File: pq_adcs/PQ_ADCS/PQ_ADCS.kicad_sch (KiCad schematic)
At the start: 55 parts, among them J1 CES-110-02-L-S, J10 Pico-Clasp_01x09, J11 Pico-Clasp_01x15, J12 CES-102-02-L-S, J2 CES-110-02-L-S, J3 CES-110-02-L-S, J4 CES-110-02-L-S, J5 Pico-Clasp_01x02, J6 Pico-Clasp_01x10, J7 Pico-Clasp_01x10, J8 Pico-Clasp_01x10, J9 Pico-Clasp_01x10, U1 LPV542, U2 LPV542, U3 LPV542, U4 IIM-42652, U5 TLC59208FIRGYR, U6 TMUX1108RSVR, U7 TCN75AVOA713

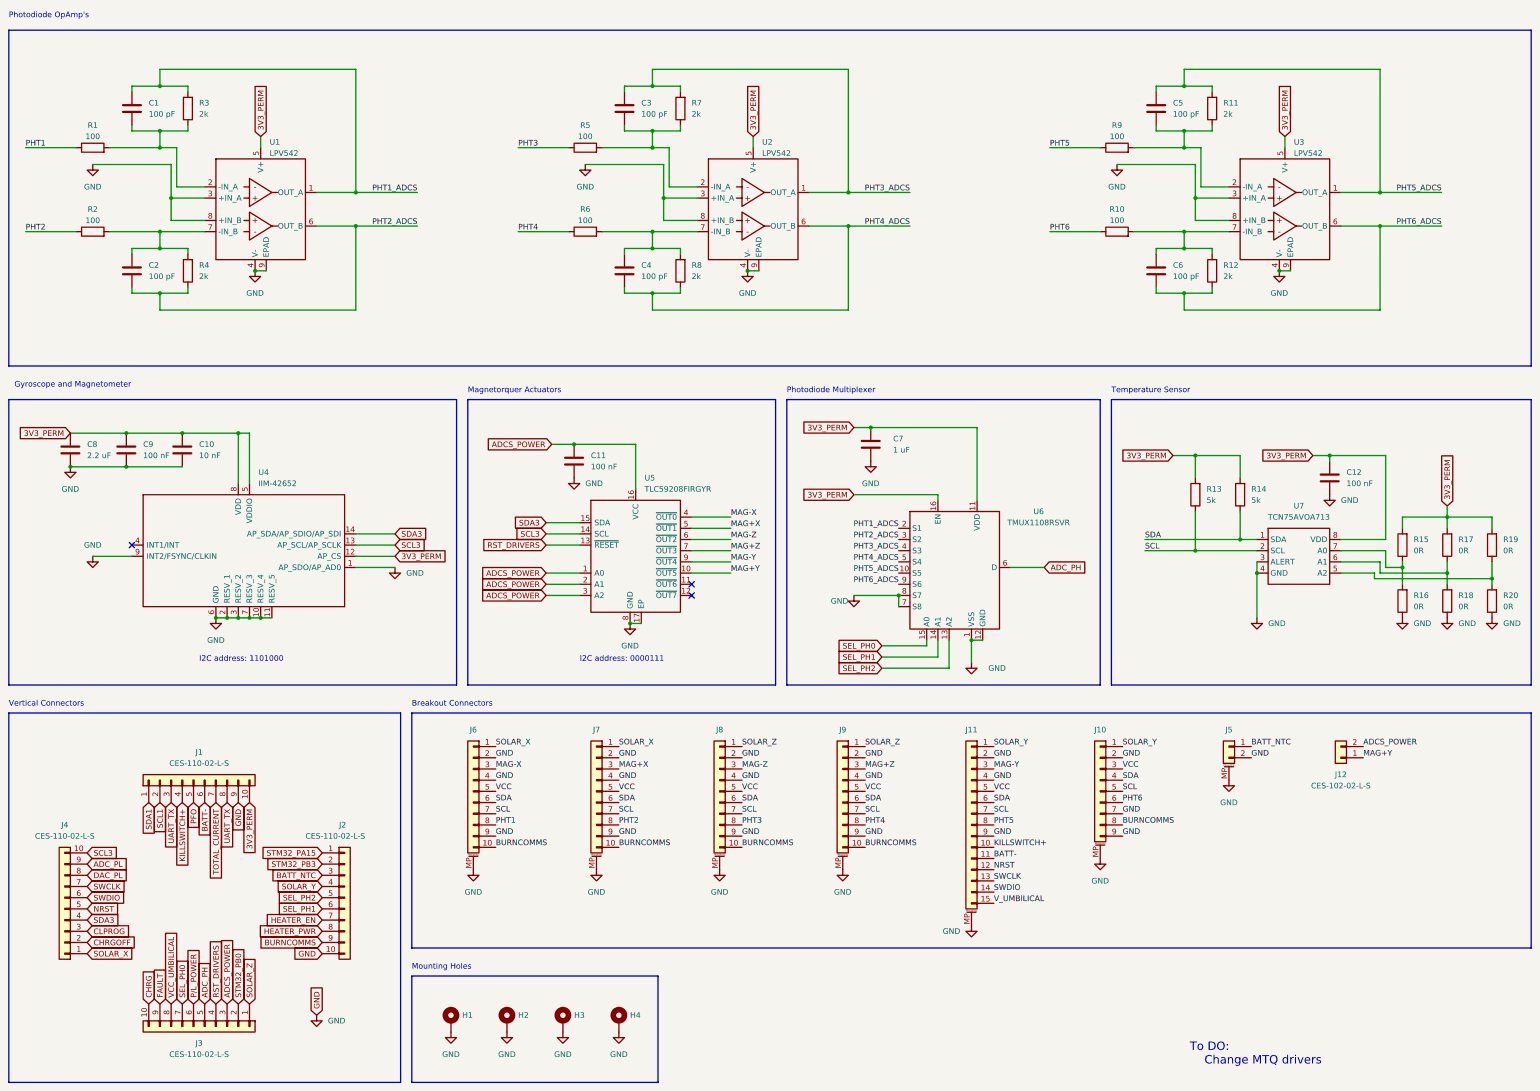
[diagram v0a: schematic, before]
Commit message: designs updated
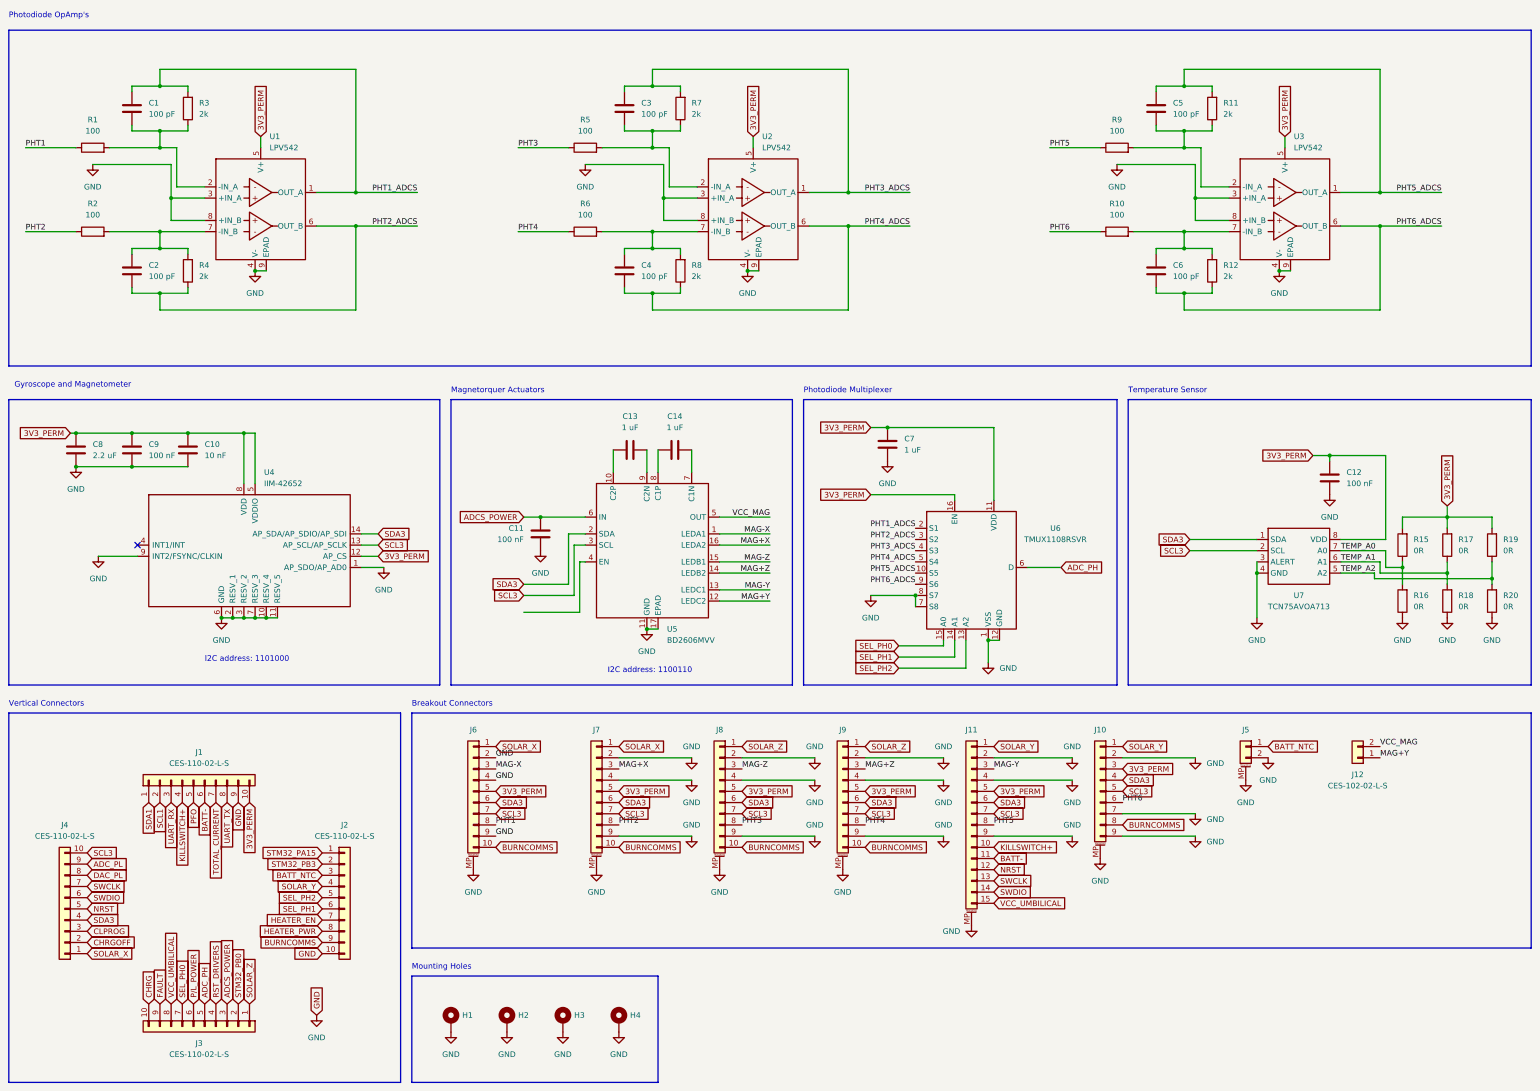
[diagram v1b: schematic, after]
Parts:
- removed R13, R14: 5k, Resistor_SMD:R_0603_1608Metric, symbol Device:R
- removed U5: TLC59208FIRGYR, symbol SamacSys_Parts:TLC59208FIRGYR
- added C13, C14: 1 uF, Capacitor_SMD:C_0603_1608Metric, symbol Device:C
- added U5: BD2606MVV, Package_DFN_QFN:QFN-16-1EP_4x4mm_P0.65mm_EP2.5x2.5mm, symbol GGS_Miscellaneous:BD2606MVV
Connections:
- net SCL is gone; now on net SCL3: J10.5 (Pin_5), J11.7 (Pin_7), J6.7 (Pin_7), J7.7 (Pin_7), J8.7 (Pin_7), J9.7 (Pin_7), U7.2 (SCL)
- net SDA is gone; now on net SDA3: J10.4 (Pin_4), J11.6 (Pin_6), J6.6 (Pin_6), J7.6 (Pin_6), J8.6 (Pin_6), J9.6 (Pin_6), U7.1 (SDA)
- net VCC is gone; now on net 3V3_PERM: J10.3 (Pin_3), J11.5 (Pin_5), J6.5 (Pin_5), J7.5 (Pin_5), J8.5 (Pin_5), J9.5 (Pin_5)
- net V_UMBILICAL is gone; now on net VCC_UMBILICAL: J11.15 (Pin_15)
- net ADCS_POWER: now also U5.6 (IN); no longer J12.2 (Pin_2)
- net GND: now also U5.11 (GND), U5.17 (EPAD)
- net MAG+X: now also U5.16 (LEDA2)
- net MAG+Y: now also U5.12 (LEDC2)
- net MAG+Z: now also U5.14 (LEDB2)
- net MAG-X: now also U5.1 (LEDA1)
- net MAG-Y: now also U5.13 (LEDC1)
- net MAG-Z: now also U5.15 (LEDB1)
- net SCL3: now also U5.3 (SCL)
- net SDA3: now also U5.2 (SDA)
- net UART_TX: no longer J1.3 (Pin_3)
- net TEMP_A2: now reaches R19.1, R20.2, U7.5 (A2)
- net TEMP_A1: now reaches R17.1, R18.2, U7.6 (A1)
- net TEMP_A0: now reaches R15.1, R16.2, U7.7 (A0)
- new net: C13.1, U5.10 (C2P)
- new net: C13.2, U5.9 (C2N)
- new net: C14.1, U5.8 (C1P)
- new net: C14.2, U5.7 (C1N)
- new net UART_RX: J1.3 (Pin_3)
- new net VCC_MAG: J12.2 (Pin_2), U5.5 (OUT)
- no-connect marks 3 -> 1
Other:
- note added: "I2C address: 1100110"
- note removed: "I2C address: 0000111"
- note removed: "To DO: Change MTQ drivers"
- moved on the sheet: C10, C7, C8, C9, J12, J5, U4, U6

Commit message: lots of changes
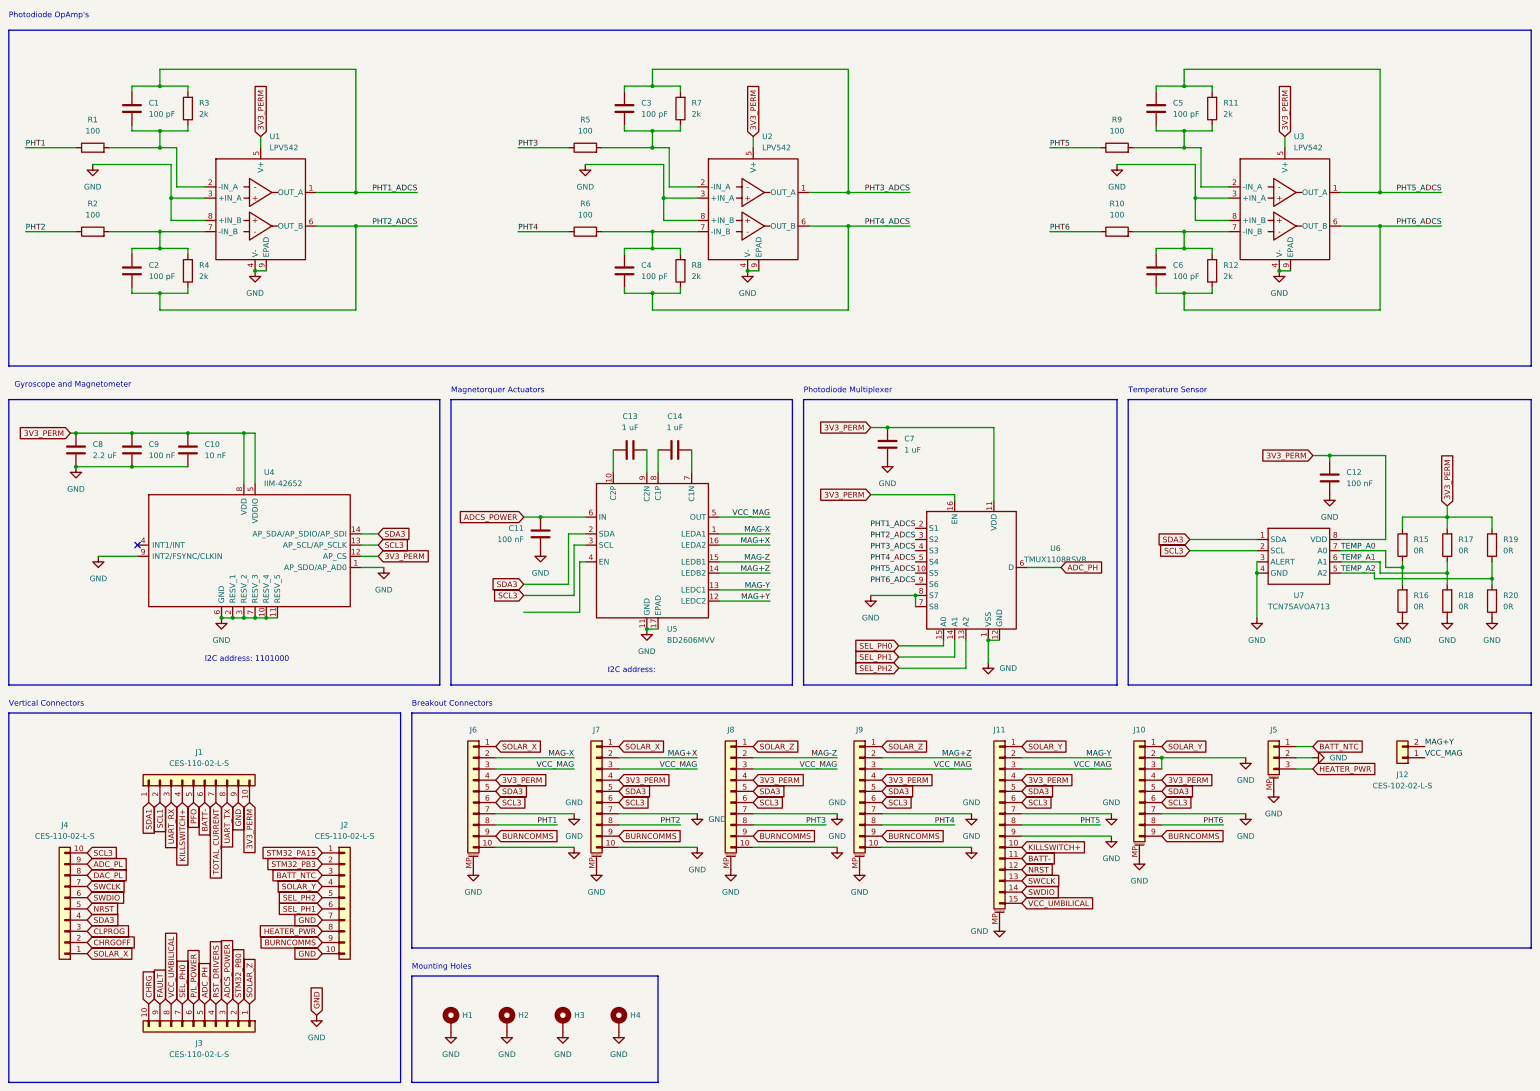
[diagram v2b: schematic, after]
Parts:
- removed J5: Pico-Clasp_01x02, Connector_Molex:Molex_Pico-Clasp_202396-0207_1x02-1MP_P1.00mm_Horizontal, symbol Connector_Generic_MountingPin:Conn_01x02_MountingPin
- added J5: Conn_01x03_MountingPin, symbol Connector_Generic_MountingPin:Conn_01x03_MountingPin
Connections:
- net HEATER_EN is gone; now on net GND: J2.7 (Pin_7)
- net 3V3_PERM: now also J10.4 (Pin_4), J11.4 (Pin_4), J6.4 (Pin_4), J7.4 (Pin_4), J8.4 (Pin_4), J9.4 (Pin_4); no longer J10.3 (Pin_3), J11.5 (Pin_5), J6.5 (Pin_5), J7.5 (Pin_5), J8.5 (Pin_5), J9.5 (Pin_5)
- net BATT_NTC: now also J5.1 (Pin_1)
- net BURNCOMMS: now also J10.9 (Pin_9), J6.9 (Pin_9), J7.9 (Pin_9), J8.9 (Pin_9), J9.9 (Pin_9); no longer J10.8 (Pin_8), J6.10 (Pin_10), J7.10 (Pin_10), J8.10 (Pin_10), J9.10 (Pin_10)
- net GND: now also J10.3 (Pin_3), J11.7 (Pin_7), J6.10 (Pin_10), J6.7 (Pin_7), J7.10 (Pin_10), J7.7 (Pin_7), J8.10 (Pin_10), J8.7 (Pin_7), J9.10 (Pin_10), J9.7 (Pin_7), J5.2 (Pin_2), J5.MP (MountPin); no longer J10.9 (Pin_9), J11.2 (Pin_2), J11.4 (Pin_4), J6.2 (Pin_2), J6.4 (Pin_4), J6.9 (Pin_9), J7.2 (Pin_2), J7.4 (Pin_4), J7.9 (Pin_9), J8.2 (Pin_2), J8.4 (Pin_4), J8.9 (Pin_9), J9.2 (Pin_2), J9.4 (Pin_4), J9.9 (Pin_9)
- net HEATER_PWR: now also J5.3 (Pin_3)
- net MAG+X: now also J7.2 (Pin_2); no longer J7.3 (Pin_3)
- net MAG+Y: now also J12.2 (Pin_2); no longer J12.1 (Pin_1)
- net MAG+Z: now also J9.2 (Pin_2); no longer J9.3 (Pin_3)
- net MAG-X: now also J6.2 (Pin_2); no longer J6.3 (Pin_3)
- net MAG-Y: now also J11.2 (Pin_2); no longer J11.3 (Pin_3)
- net MAG-Z: now also J8.2 (Pin_2); no longer J8.3 (Pin_3)
- net PHT6: now also J10.8 (Pin_8); no longer J10.6 (Pin_6)
- net SCL3: now also J10.6 (Pin_6), J11.6 (Pin_6), J6.6 (Pin_6), J7.6 (Pin_6), J8.6 (Pin_6), J9.6 (Pin_6); no longer J10.5 (Pin_5), J11.7 (Pin_7), J6.7 (Pin_7), J7.7 (Pin_7), J8.7 (Pin_7), J9.7 (Pin_7)
- net SDA3: now also J10.5 (Pin_5), J11.5 (Pin_5), J6.5 (Pin_5), J7.5 (Pin_5), J8.5 (Pin_5), J9.5 (Pin_5); no longer J10.4 (Pin_4), J11.6 (Pin_6), J6.6 (Pin_6), J7.6 (Pin_6), J8.6 (Pin_6), J9.6 (Pin_6)
- net VCC_MAG: now also J11.3 (Pin_3), J12.1 (Pin_1), J6.3 (Pin_3), J7.3 (Pin_3), J8.3 (Pin_3), J9.3 (Pin_3); no longer J12.2 (Pin_2)
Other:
- note added: "I2C address:"
- note removed: "I2C address: 1100110"
- moved on the sheet: J10, J11, J12, J8, J9

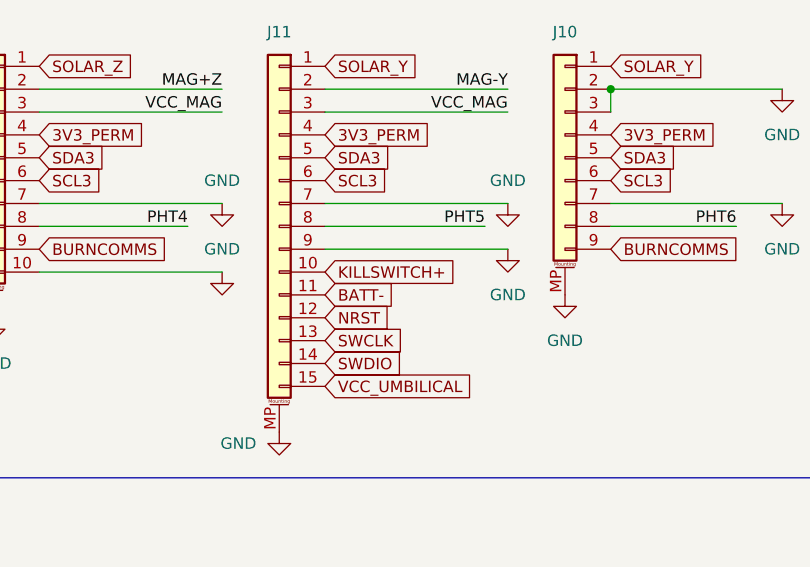
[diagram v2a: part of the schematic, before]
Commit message: adcs board ready for manufacturing
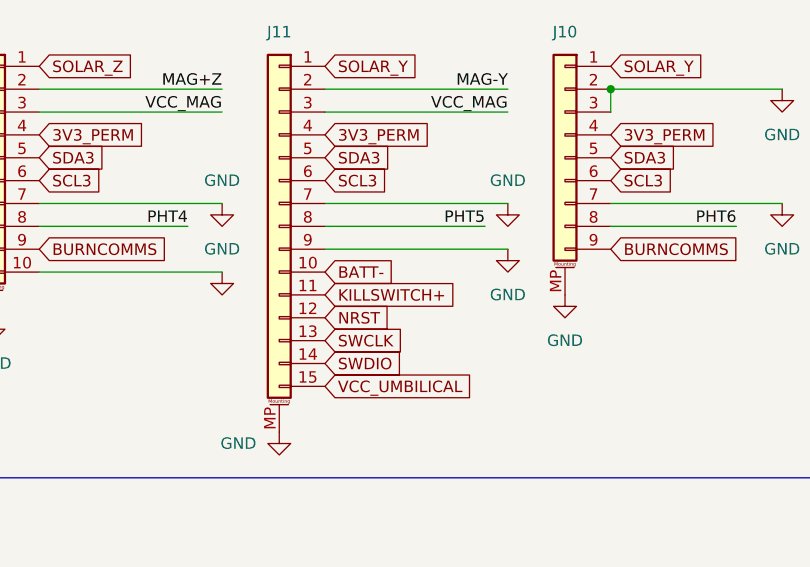
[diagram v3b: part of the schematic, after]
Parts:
- J5: footprint (none) -> Connector_Molex:Molex_Pico-Clasp_202396-0307_1x03-1MP_P1.00mm_Horizontal
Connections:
- net BATT-: now also J11.10 (Pin_10); no longer J11.11 (Pin_11)
- net KILLSWITCH+: now also J11.11 (Pin_11); no longer J11.10 (Pin_10)
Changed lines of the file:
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@@
+    )
+  )
+  (global_label "BATT-" (shape input) (at 264.16 214.63 0) (fields_autoplaced)
+    (effects (font (size 1.27 1.27)) (justify left))
+    (property "Intersheet References" "${INTERSHEET_REFS}" (id 0) (at 272.4393 214.5506 0)
+      (effects (font (size 1.27 1.27)) (justify left) hide)
     )
   )
@@
     )
   )
-  (global_label "BATT-" (shape input) (at 264.16 217.17 0) (fields_autoplaced)
-    (effects (font (size 1.27 1.27)) (justify left))
-    (property "Intersheet References" "${INTERSHEET_REFS}" (id 0) (at 272.4393 217.0906 0)
-      (effects (font (size 1.27 1.27)) (justify left) hide)
-    )
-  )
   (global_label "SDA3" (shape input) (at 264.16 201.93 0) (fields_autoplaced)
     (effects (font (size 1.27 1.27)) (justify left))
@@
     )
   )
+  (global_label "KILLSWITCH+" (shape input) (at 264.16 217.17 0) (fields_autoplaced)
+    (effects (font (size 1.27 1.27)) (justify left))
+    (property "Intersheet References" "${INTERSHEET_REFS}" (id 0) (at 278.9102 217.0906 0)
+      (effects (font (size 1.27 1.27)) (justify left) hide)
+    )
+  )
   (global_label "GND" (shape input) (at 104.14 252.73 90) (fields_autoplaced)
     (effects (font (size 1.27 1.27)) (justify left))
@@
     (effects (font (size 1.27 1.27)) (justify left))
     (property "Intersheet References" "${INTERSHEET_REFS}" (id 0) (at 71.0406 233.5045 90)
-      (effects (font (size 1.27 1.27)) (justify left) hide)
-    )
-  )
-  (global_label "KILLSWITCH+" (shape input) (at 264.16 214.63 0) (fields_autoplaced)
-    (effects (font (size 1.27 1.27)) (justify left))
-    (property "Intersheet References" "${INTERSHEET_REFS}" (id 0) (at 278.9102 214.5506 0)
       (effects (font (size 1.27 1.27)) (justify left) hide)
     )
@@
       (effects (font (size 1.27 1.27)) hide)
     )
-    (property "Footprint" "" (id 2) (at 321.31 194.31 0)
-      (effects (font (size 1.27 1.27)) hide)
-    )
+    (property "Footprint" "Connector_Molex:Molex_Pico-Clasp_202396-0307_1x03-1MP_P1.00mm_Horizontal" (id 2) (at 321.31 194.31 0)
+      (effects (font (size 1.27 1.27)) hide)
+    )

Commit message: BoM
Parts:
- C1, C2, C3, C4, C5, C6: Manufacturer 1 (none) -> KYOCERA AVX; Manufacturer Part Number 1 (none) -> 06035C101K4T2A; Supplier 1 (none) -> Mouser; Supplier Part Number 1 (none) -> 581-06035C101K4T2A
- J5: value Conn_01x03_MountingPin -> Pico-Clasp_01x03; Manufacturer 1 (none) -> Molex; Manufacturer Part Number 1 (none) -> 203556-0307; Supplier 1 (none) -> Mouser; Supplier Part Number 1 (none) -> 538-203556-0307
- R1, R10, R2, R5, R6, R9: Manufacturer 1 (none) -> YAGEO; Manufacturer Part Number 1 (none) -> AC0603FR-13100RL; Supplier 1 (none) -> Mouser; Supplier Part Number 1 (none) -> 603-AC0603FR-13100RL
- R11, R12, R3, R4, R7, R8: Manufacturer 1 (none) -> YAGEO; Manufacturer Part Number 1 (none) -> RC0603FR-132KL; Supplier 1 (none) -> Mouser; Supplier Part Number 1 (none) -> 603-RC0603FR-132KL
- R15, R16, R17, R18, R19, R20: Manufacturer 1 (none) -> Bourns; Manufacturer Part Number 1 (none) -> CR0402AJ/-000GAS; Supplier 1 (none) -> Mouser; Supplier Part Number 1 (none) -> 652-CR0402AJ/-000GAS
- U5: Manufacturer 1 (none) -> ROHM Semiconductor; Manufacturer Part Number 1 (none) -> BD2606MVV-E2; Supplier 1 (none) -> Mouser; Supplier Part Number 1 (none) -> 755-BD2606MVV-E2
